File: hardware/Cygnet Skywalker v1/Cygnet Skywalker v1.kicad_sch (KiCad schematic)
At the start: 0 parts

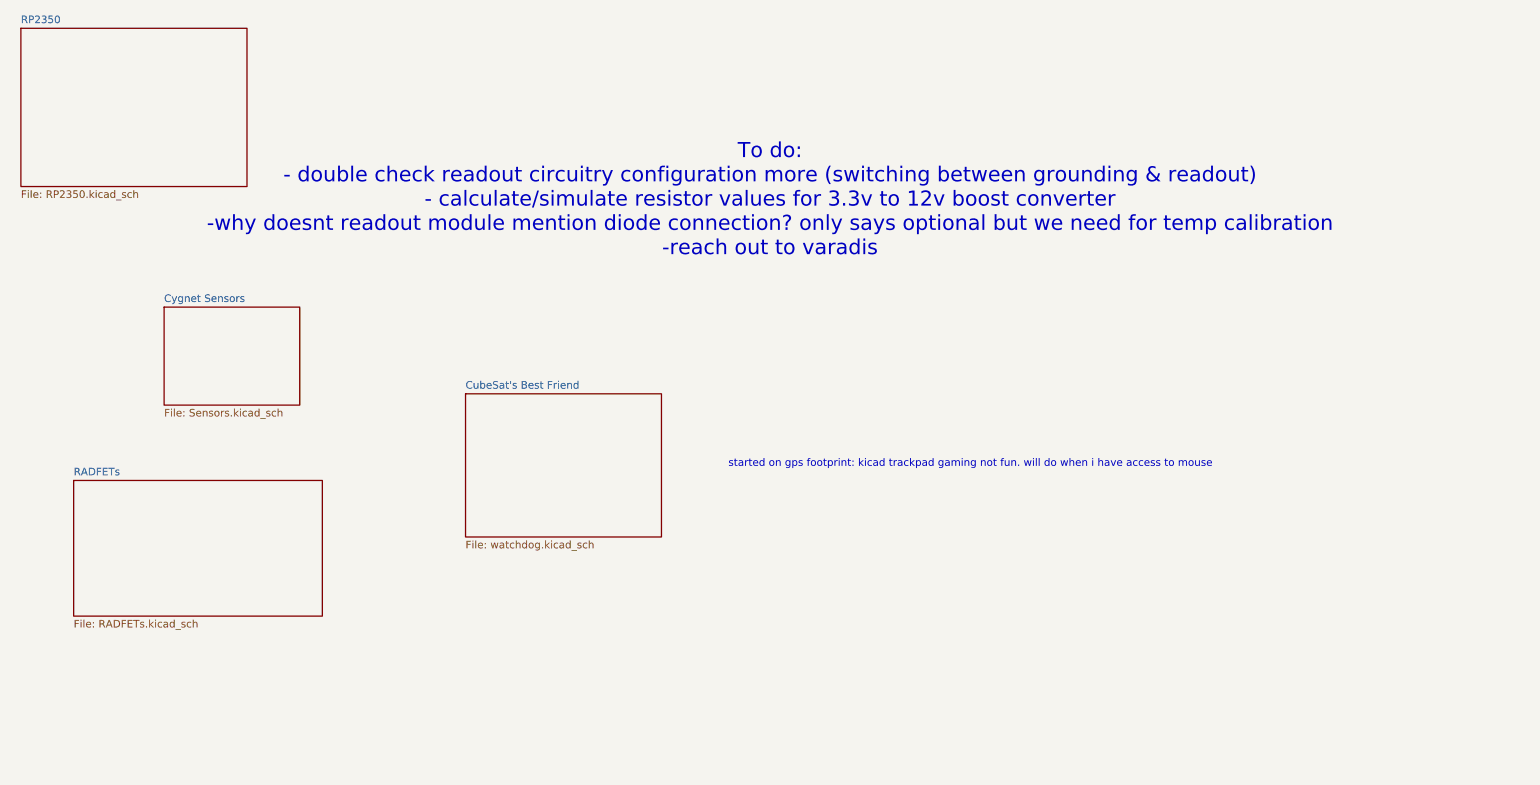
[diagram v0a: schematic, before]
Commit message: final schematic used for layout
layout yay
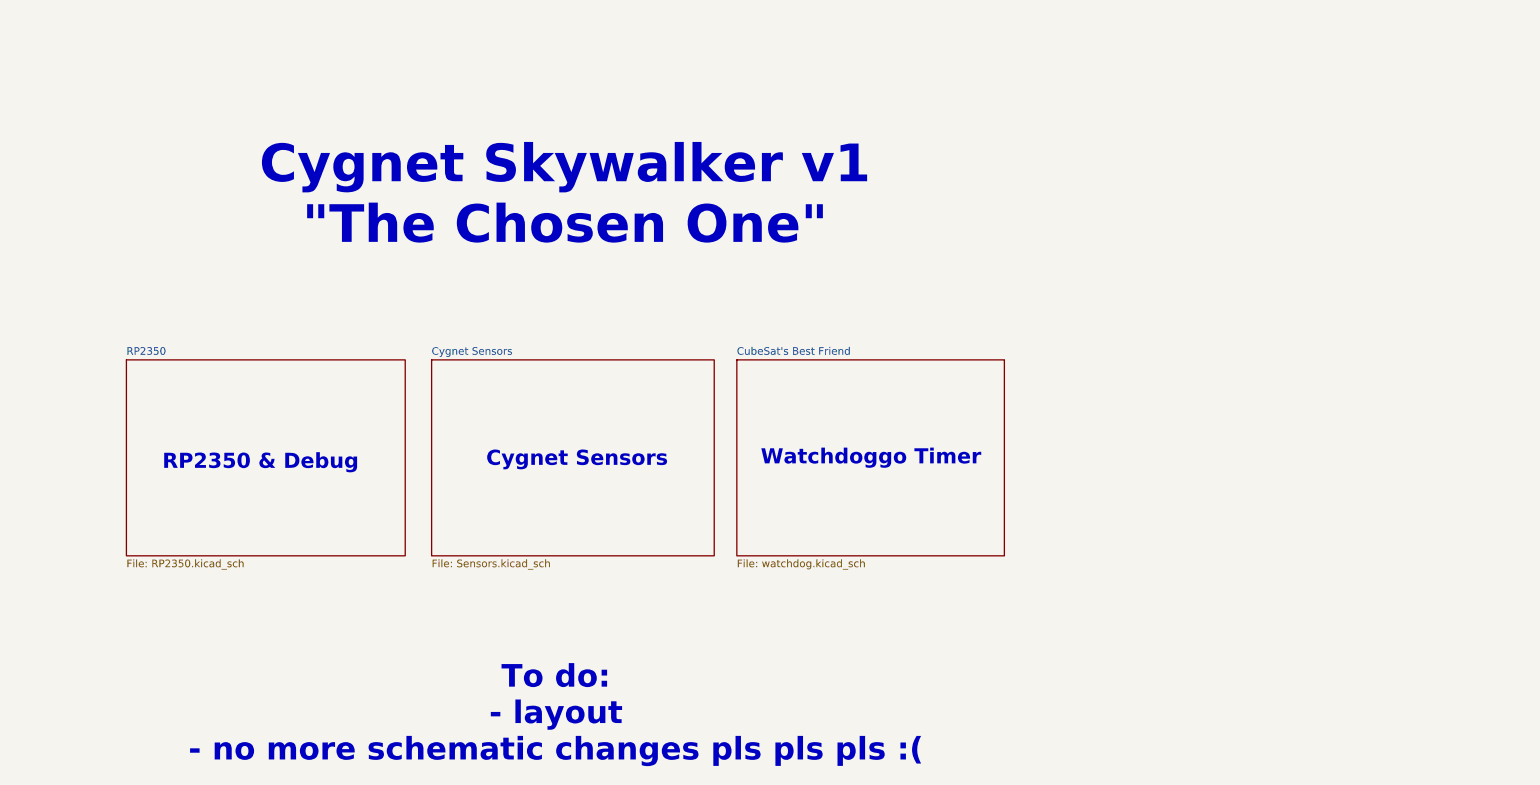
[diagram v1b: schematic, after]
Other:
- removed sheet RADFETs
- note added: "Cygnet Sensors"
- note added: "Cygnet Skywalker v1 "The Chosen One""
- note added: "RP2350 & Debug"
- note added: "To do: - layout - no more schematic changes pls pls pls :("
- note added: "Watchdoggo Timer"
- note removed: "To do: - double check readout circuitry configuration more (switching between grounding & readout) - calculate/simulate resistor values for 3.3v to 12v boost converter -why doesnt readout module mention diode connection? only says optional but we need for temp calibration -reach out to varadis"
- note removed: "started on gps footprint: kicad trackpad gaming not fun. will do when i have access to mouse"
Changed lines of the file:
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@@
 	(generator_version "9.0")
 	(paper "A4")
-	(text "started on gps footprint: kicad trackpad gaming not fun. will do when i have access to mouse"
+	(text "Cygnet Skywalker v1\n\"The Chosen One\""
 		(exclude_from_sim no)
-		(at 213.36 105.156 0)
+		(at 145.034 59.944 0)
 		(effects
 			(font
-				(size 1.27 1.27)
+				(size 6.35 6.35)
+				(thickness 1.016)
+				(bold yes)
 			)
 		)
 	)
-	(text "To do:\n- double check readout circuitry configuration more (switching between grounding & readout)\n- calculate/simulate resistor values for 3.3v to 12v boost converter\n-why doesnt readout module mention diode connection? only says optional but we need for temp calibration\n-reach out to varadis"
+	(text "Cygnet Sensors"
 		(exclude_from_sim no)
-		(at 179.578 60.706 0)
+		(at 147.066 104.394 0)
 		(effects
 			(font
 				(size 2.54 2.54)
+				(thickness 0.254)
+				(bold yes)
+			)
+		)
+	)
+	(text "Watchdoggo Timer"
+		(exclude_from_sim no)
+		(at 196.596 104.14 0)
+		(effects
+			(font
+				(size 2.54 2.54)
+				(thickness 0.254)
+				(bold yes)
+			)
+		)
+	)
+	(text "To do:\n- layout\n- no more schematic changes pls pls pls :("
+		(exclude_from_sim no)
+		(at 143.51 147.32 0)
+		(effects
+			(font
+				(size 3.81 3.81)
+				(thickness 0.762)
+				(bold yes)
+			)
+		)
+	)
+	(text "RP2350 & Debug"
+		(exclude_from_sim no)
+		(at 93.726 104.902 0)
+		(effects
+			(font
+				(size 2.54 2.54)
+				(thickness 0.254)
+				(bold yes)
 			)
 		)
 	)
 	(sheet
-		(at 77.47 78.74)
-		(size 22.86 16.51)
+		(at 122.555 87.63)
+		(size 47.625 33.02)
 		(exclude_from_sim no)
 		(in_bom yes)
@@
 		)
 		(property "Sheetname" "Cygnet Sensors"
-			(at 77.47 78.0284 0)
+			(at 122.555 86.9184 0)
 			(effects
 				(font
@@
 		)
 		(property "Sheetfile" "Sensors.kicad_sch"
-			(at 77.47 95.8346 0)
+			(at 122.555 121.2346 0)
 			(effects
 				(font
@@
 	)
 	(sheet
-		(at 53.34 31.75)
-		(size 38.1 26.67)
+		(at 71.12 87.63)
+		(size 46.99 33.02)
 		(exclude_from_sim no)
 		(in_bom yes)
@@
 		)
 		(property "Sheetname" "RP2350"
-			(at 53.34 31.0384 0)
+			(at 71.12 86.9184 0)
 			(effects
 				(font
@@
 		)
 		(property "Sheetfile" "RP2350.kicad_sch"
-			(at 53.34 59.0046 0)
+			(at 71.12 121.2346 0)
 			(effects
 				(font
@@
 	)
 	(sheet
-		(at 62.23 107.95)
-		(size 41.91 22.86)
-		(exclude_from_sim no)
-		(in_bom yes)
-		(on_board yes)
-		(dnp no)
-		(fields_autoplaced yes)
-		(stroke
-			(width 0.1524)
-			(type solid)
-		)
-		(fill
-			(color 0 0 0 0.0000)
-		)
-		(property "Sheetname" "RADFETs"
-			(at 62.23 107.2384 0)
-			(effects
-				(font
-					(size 1.27 1.27)
-				)
-				(justify left bottom)
-			)
-		)
-		(property "Sheetfile" "RADFETs.kicad_sch"
-			(at 62.23 131.3946 0)
-			(effects
-				(font
-					(size 1.27 1.27)
-				)
-				(justify left top)
-			)
-		)
-		(instances
-			(project "Cygnet Skywalker v1"
-				(path "/f674abc6-f811-4b69-a04b-9059ca6b6a44"
-					(page "4")
-				)
-			)
-		)
-	)
-	(sheet
-		(at 128.27 93.345)
-		(size 33.02 24.13)
+		(at 173.99 87.63)
+		(size 45.085 33.02)
 		(exclude_from_sim no)
 		(in_bom yes)
@@
 		)
 		(property "Sheetname" "CubeSat's Best Friend"
-			(at 128.27 92.6334 0)
+			(at 173.99 86.9184 0)
 			(effects
 				(font
@@
 		)
 		(property "Sheetfile" "watchdog.kicad_sch"
-			(at 128.27 118.0596 0)
+			(at 173.99 121.2346 0)
 			(effects
 				(font
